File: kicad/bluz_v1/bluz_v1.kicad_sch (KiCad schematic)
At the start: 59 parts, among them J1 USB_B_Micro, J11 Conn, J12 BTAnt, J2 Conn, J3 Conn, J4 Conn, J5 Conn, J6 Conn, J7 Conn, J8 Conn, M1 VibroMotor, Q1 RUM002N05, Q2 RUM002N05, SW1 SW_DPDT_x2, U1 MCP73831, U2 MCP1703, U3 TLV3201AIDCK, Y1 NX2016SA-32MHz

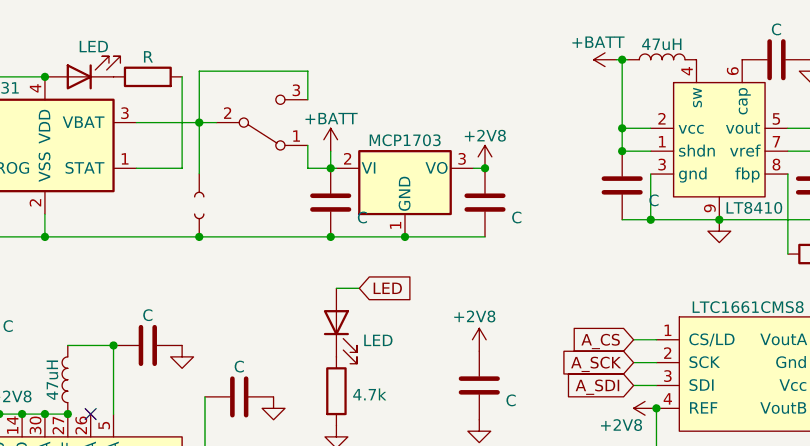
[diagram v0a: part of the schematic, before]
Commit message: изменено:      kicad/bluz_v1/bluz_v1.kicad_pcb 	изменено:      kicad/bluz_v1/bluz_v1.kicad_prl 	изменено:      kicad/bluz_v1/bluz_v1.kicad_sch
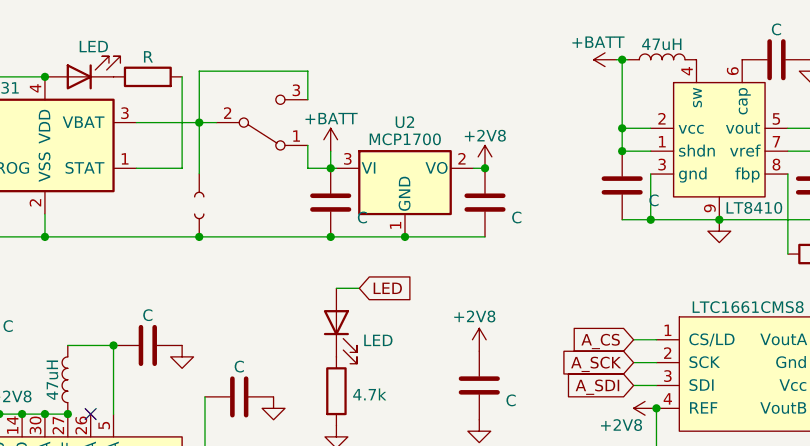
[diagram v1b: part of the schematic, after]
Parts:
- removed U2: MCP1703, Package_TO_SOT_SMD:SOT-23W, symbol Regulator_Linear:MCP1703Ax-180xxMB
- added U2: MCP1700, Package_TO_SOT_SMD:SOT-23, symbol Regulator_Linear:MCP1700x-280xxTT
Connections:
- net +2V8: now also U2.2 (VO)
- net +BATT: now also U2.3 (VI)
- net GND: now also U2.1 (GND)
